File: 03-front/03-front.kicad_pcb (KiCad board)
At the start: 2 copper layers, 120 x 23.7 mm, 18 parts, among them J1 Conn_01x10

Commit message: がんばる
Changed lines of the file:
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@@
     (fp_line (start 1.6 0.8) (end -1.6 0.8)
       (stroke (width 0.1) (type solid)) (layer "F.Fab"))
-    (pad "1" smd roundrect (at -1.4625 0 270) (size 1.125 1.75) (layers "F.Cu" "F.Paste" "F.Mask") (roundrect_rratio 0.222222)
+    (pad "1" smd roundrect (at -1.4625 0 270) (size 1.125 1.75) (layers "F.Cu" "F.Paste" "F.Mask") (roundrect_rratio 0.2222222222)
       (net 1 "+3V3") (pintype "passive"))
-    (pad "2" smd roundrect (at 1.4625 0 270) (size 1.125 1.75) (layers "F.Cu" "F.Paste" "F.Mask") (roundrect_rratio 0.222222)
+    (pad "2" smd roundrect (at 1.4625 0 270) (size 1.125 1.75) (layers "F.Cu" "F.Paste" "F.Mask") (roundrect_rratio 0.2222222222)
       (net 2 "photo1") (pintype "passive"))
     (model "${KICAD6_3DMODEL_DIR}/Resistor_SMD.3dshapes/R_1206_3216Metric.wrl"
@@
     (fp_line (start 1 0.625) (end -1 0.625)
       (stroke (width 0.1) (type solid)) (layer "F.Fab"))
-    (pad "1" smd roundrect (at -0.9125 0) (size 1.025 1.4) (layers "F.Cu" "F.Paste" "F.Mask") (roundrect_rratio 0.243902)
+    (pad "1" smd roundrect (at -0.9125 0) (size 1.025 1.4) (layers "F.Cu" "F.Paste" "F.Mask") (roundrect_rratio 0.243902439)
       (net 11 "Net-(D1-A)") (pintype "passive"))
-    (pad "2" smd roundrect (at 0.9125 0) (size 1.025 1.4) (layers "F.Cu" "F.Paste" "F.Mask") (roundrect_rratio 0.243902)
+    (pad "2" smd roundrect (at 0.9125 0) (size 1.025 1.4) (layers "F.Cu" "F.Paste" "F.Mask") (roundrect_rratio 0.243902439)
       (net 1 "+3V3") (pintype "passive"))
     (model "${KICAD6_3DMODEL_DIR}/Resistor_SMD.3dshapes/R_0805_2012Metric.wrl"
@@
     (pad "9" thru_hole oval (at 0 -20.32 270) (size 1.7 1.7) (drill 1) (layers "*.Cu" "*.Mask"))
     (pad "10" thru_hole oval (at 0 -22.86 270) (size 1.7 1.7) (drill 1) (layers "*.Cu" "*.Mask"))
-    (model "${KICAD6_3DMODEL_DIR}/Connector_PinHeader_2.54mm.3dshapes/PinHeader_1x10_P2.54mm_Horizontal.wrl"
+    (model "${KICAD6_3DMODEL_DIR}/Connector_PinHeader_2.54mm.3dshapes/PinHeader_1x10_P2.54mm_Horizontal.wrl" hide
       (offset (xyz 0 0 0))
       (scale (xyz 1 1 1))
@@
     (pad "10" thru_hole oval (at 0 -22.86 270) (size 1.7 1.7) (drill 1) (layers "*.Cu" "*.Mask")
       (net 3 "GND") (pinfunction "Pin_10") (pintype "passive"))
-    (model "${KICAD6_3DMODEL_DIR}/Connector_PinHeader_2.54mm.3dshapes/PinHeader_1x10_P2.54mm_Horizontal.wrl"
+    (model "${KICAD6_3DMODEL_DIR}/Connector_PinHeader_2.54mm.3dshapes/PinHeader_1x10_P2.54mm_Horizontal.wrl" hide
       (offset (xyz 0 0 0))
       (scale (xyz 1 1 1))

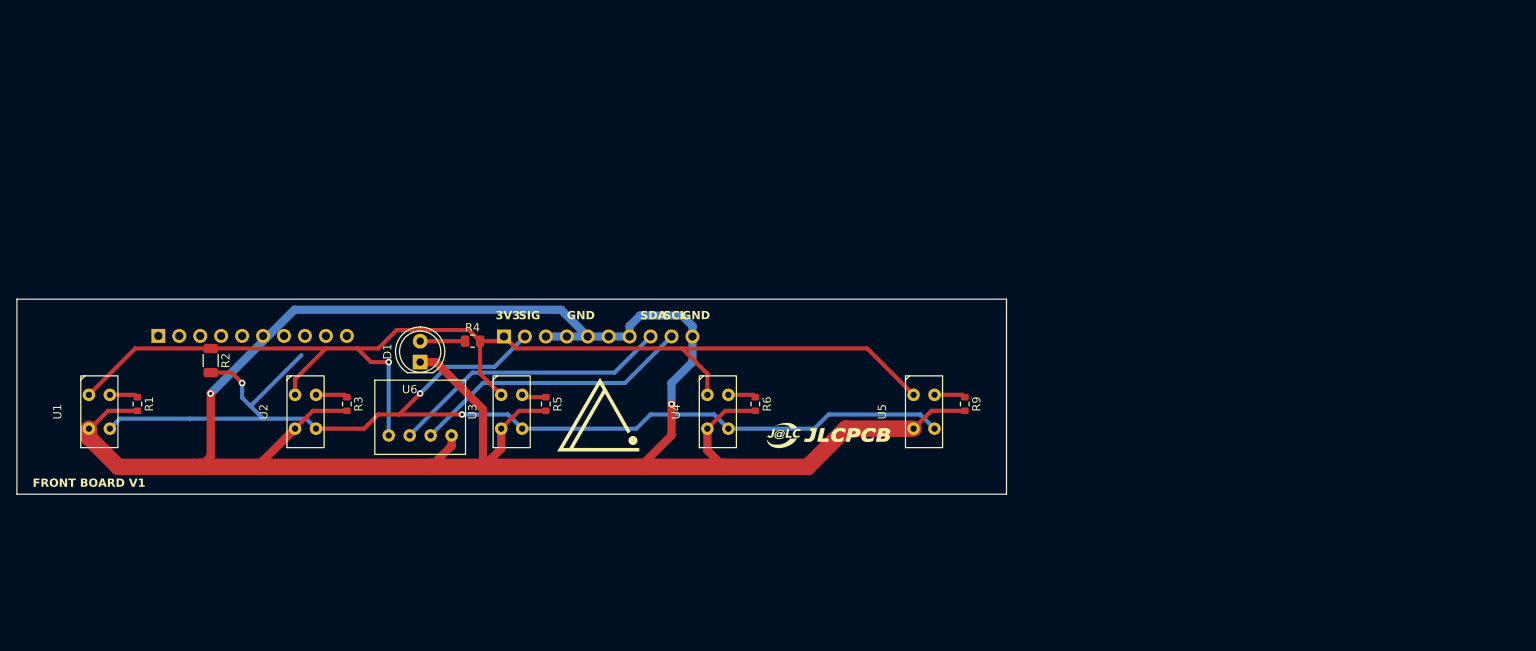
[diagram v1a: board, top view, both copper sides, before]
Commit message: わああ
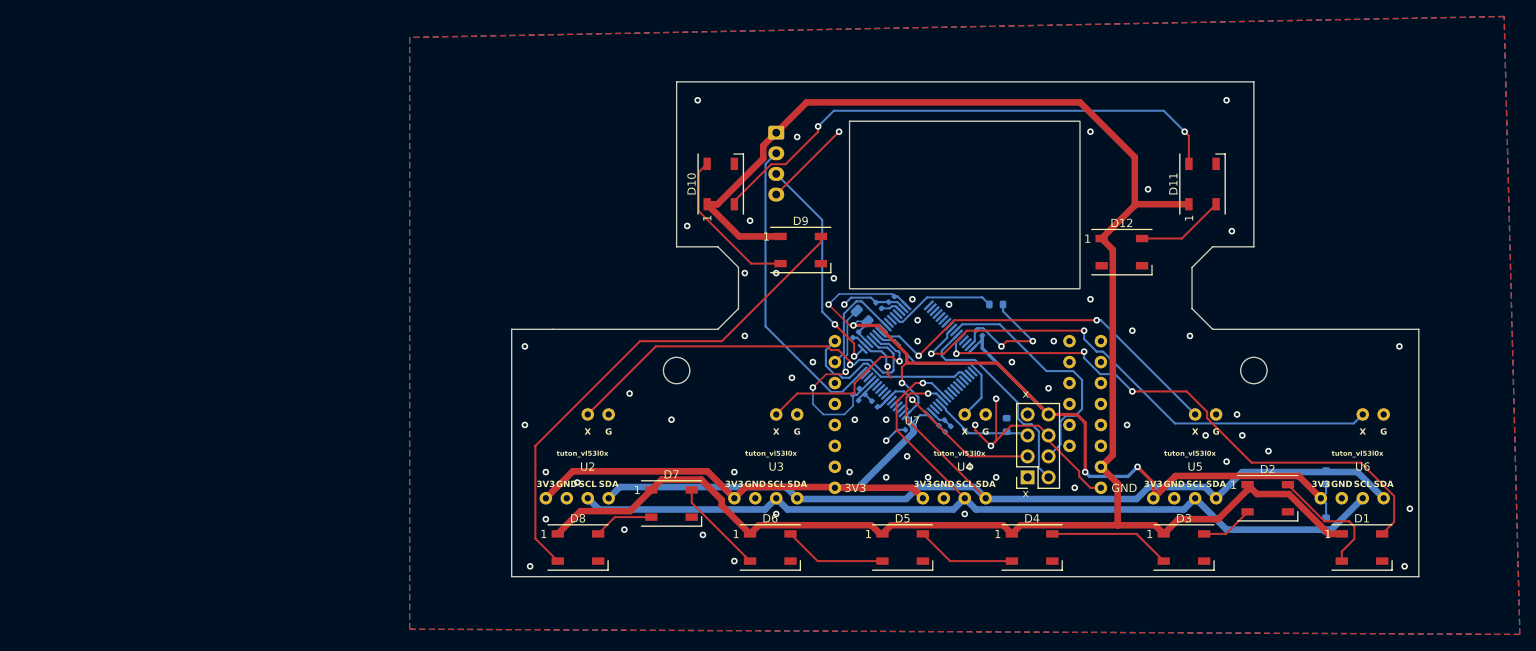
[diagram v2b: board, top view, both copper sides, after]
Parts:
- removed the G*** at (138.4, 102.9)
- removed R5, R6, R9: 105, Resistor_SMD:R_0603_1608Metric
- removed the REF** at (57.1, 90.8)
- added C1: 100n, Capacitor_SMD:C_0402_1005Metric, B.Cu at (144.0, 99.1)
- added C10: 1u, Capacitor_SMD:C_0402_1005Metric, B.Cu at (141.7, 98.3)
- added C2: 4.7u, Capacitor_SMD:C_0402_1005Metric, B.Cu at (144.5, 87.1)
- added C3: 100n, Capacitor_SMD:C_0402_1005Metric, B.Cu at (156.7, 90.4)
- added C4: 100n, Capacitor_SMD:C_0402_1005Metric, B.Cu at (141.7, 90.7)
- added C5: 100n, Capacitor_SMD:C_0402_1005Metric, B.Cu at (148.1, 101.9)
- added C6: 100n, Capacitor_SMD:C_0402_1005Metric, B.Cu at (146.1, 86.4)
- added C7: 4.7u, Capacitor_SMD:C_0402_1005Metric, B.Cu at (152.9, 102.1)
- added C8: 100n, Capacitor_SMD:C_0402_1005Metric, B.Cu at (152.1, 101.3)
- added C9: 100n, Capacitor_SMD:C_0402_1005Metric, B.Cu at (142.5, 97.5)
- added D10: WS2812B, LED_SMD:LED_WS2812B_PLCC4_5.0x5.0mm_P3.2mm, F.Cu at (125.3, 72.4)
- added D11: WS2812B, LED_SMD:LED_WS2812B_PLCC4_5.0x5.0mm_P3.2mm, F.Cu at (183.8, 72.4)
- added D12: WS2812B, LED_SMD:LED_WS2812B_PLCC4_5.0x5.0mm_P3.2mm, F.Cu at (174.0, 80.6)
- added D2: WS2812B, LED_SMD:LED_WS2812B_PLCC4_5.0x5.0mm_P3.2mm, F.Cu at (191.7, 110.5)
- added D3: WS2812B, LED_SMD:LED_WS2812B_PLCC4_5.0x5.0mm_P3.2mm, F.Cu at (181.5, 116.5)
- added D4: WS2812B, LED_SMD:LED_WS2812B_PLCC4_5.0x5.0mm_P3.2mm, F.Cu at (163.1, 116.5)
- added D5: WS2812B, LED_SMD:LED_WS2812B_PLCC4_5.0x5.0mm_P3.2mm, F.Cu at (147.4, 116.5)
- added D6: WS2812B, LED_SMD:LED_WS2812B_PLCC4_5.0x5.0mm_P3.2mm, F.Cu at (131.4, 116.5)
- added D7: WS2812B, LED_SMD:LED_WS2812B_PLCC4_5.0x5.0mm_P3.2mm, F.Cu at (119.4, 111.1)
- added D8: WS2812B, LED_SMD:LED_WS2812B_PLCC4_5.0x5.0mm_P3.2mm, F.Cu at (108.0, 116.5)
- added D9: WS2812B, LED_SMD:LED_WS2812B_PLCC4_5.0x5.0mm_P3.2mm, F.Cu at (135.1, 80.4)
- added FB1: FerriteBead, Resistor_SMD:R_0805_2012Metric, B.Cu at (142.5, 88.4)
- added G***: LOGO, logo:st_logo, B.Cu at (191.8, 108.0)
- added G***: LOGO, logo:jlcpcb_logo, B.Cu at (191.8, 104.1)
- added J2: ToMAIN, Connector_JST:JST_XH_B4B-XH-A_1x04_P2.50mm_Vertical, B.Cu at (132.1, 66.2)
- added REF**: MountingHole_3.2mm_M3, MountingHole:MountingHole_3.2mm_M3, F.Cu at (190.0, 95.0)
- added REF**: MountingHole_3.2mm_M3, MountingHole:MountingHole_3.2mm_M3, F.Cu at (120.0, 95.0)
- added U7: ~, OpenMV:OpenMV h7, F.Cu at (148.6, 101.6)
- D1: value LED -> WS2812B; footprint LED_THT:LED_D5.0mm -> LED_SMD:LED_WS2812B_PLCC4_5.0x5.0mm_P3.2mm
- G***: moved to B.Cu
- J1: value Conn_01x10 -> WRITER CONN; footprint Connector_PinHeader_2.54mm:PinHeader_1x10_P2.54mm_Horizontal -> Connector_PinSocket_2.54mm:PinSocket_2x04_P2.54mm_Vertical; moved to F.Cu
- R1, R3: value 105 -> 10k; moved to B.Cu
- R2: value 1k -> 10k; footprint Resistor_SMD:R_1206_3216Metric -> Resistor_SMD:R_0603_1608Metric; moved to B.Cu
- R4: value 100 -> 10k; footprint Resistor_SMD:R_0805_2012Metric -> Resistor_SMD:R_0603_1608Metric; moved to B.Cu
- U1: value ~ -> STM32F446RETx; footprint Akiduki:LBR127HLD -> Package_QFP:LQFP-64_10x10mm_P0.5mm; moved to B.Cu
- U2, U3, U4, U5: footprint Akiduki:LBR127HLD -> tuton:VL53L0X_horizontal
- U6: footprint S11059:S11059 -> tuton:VL53L0X_horizontal
- moved R3 119.1 mm to (198.8, 108.0), turned to 90 degrees
- moved D1 116.4 mm to (203.1, 116.5), turned to 0 degrees
- moved U6 109.5 mm to (198.1, 110.5)
- moved R4 105.9 mm to (198.8, 113.7), turned to 90 degrees
- moved R1 105.4 mm to (160.0, 101.6), turned to 90 degrees
- moved U1 99.4 mm to (149.2, 93.8), turned to 45 degrees
- moved R2 95.5 mm to (158.8, 87.0), turned to 0 degrees
- moved J1 65.8 mm to (162.6, 108.0), turned to 180 degrees
- moved U2 31.0 mm to (104.1, 110.5), turned to 0 degrees
- moved U5 29.7 mm to (177.8, 110.5), turned to 0 degrees
- moved U3 29.0 mm to (127.0, 110.5), turned to 0 degrees
- moved U4 27.0 mm to (149.9, 110.5), turned to 0 degrees
- moved G*** 11.3 mm to (119.4, 107.3), turned to 180 degrees
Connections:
- D1 pad 1: GND -> +5V
- D1 pad 2: Net-(D1-A) -> Net-(D1-DOUT)
- J1 pad 1: +3V3 -> unconnected-(J1-Pin_1-Pad1)
- J1 pad 2: photo1 -> UART1_RX
- J1 pad 3: GND -> NRST
- J1 pad 4: GND -> UART1_TX
- J1 pad 5: GND -> BOOT0
- J1 pad 7: GND -> unconnected-(J1-Pin_7-Pad7)
- J1 pad 8: SDA -> +3V3
- R1 pad 1: Net-(U1-Cathode) -> BOOT0
- R2 pad 1: +3V3 -> Net-(U1-PB2)
- R2 pad 2: photo1 -> GND
- R3 pad 1: Net-(U2-Cathode) -> +3V3
- R3 pad 2: GND -> I2C1_SDA
- R4 pad 1: Net-(D1-A) -> I2C1_SCL
- U1 pad 2: Net-(U1-Cathode) -> unconnected-(U1-PC13-Pad2)
- U1 pad 3: GND -> unconnected-(U1-PC14-Pad3)
- U1 pad 4: photo1 -> unconnected-(U1-PC15-Pad4)
- U2 pad 2: Net-(U2-Cathode) -> GND
- U2 pad 3: GND -> I2C1_SCL
- U2 pad 4: photo1 -> I2C1_SDA
- U3 pad 2: Net-(U3-Cathode) -> GND
- U3 pad 3: GND -> I2C1_SCL
- U3 pad 4: photo1 -> I2C1_SDA
- U4 pad 2: Net-(U4-Cathode) -> GND
- U4 pad 3: GND -> I2C1_SCL
- U4 pad 4: photo1 -> I2C1_SDA
- U5 pad 2: Net-(U5-Cathode) -> GND
- U5 pad 3: GND -> I2C1_SCL
- U5 pad 4: photo1 -> I2C1_SDA
- U6 pad 2: SDA -> GND
- U6 pad 3: SCL -> I2C1_SCL
- U6 pad 4: GND -> I2C1_SDA
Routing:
- net +5V: track 0.00 -> 234.9 mm
- net GND: track 278.1 -> 80.3 mm, vias 2 -> 65
- net photo1: track 142.9 -> 0.00 mm, vias 3 -> 0
- net I2C1_SCL: track 0.00 -> 123.3 mm, vias 0 -> 1
- net I2C1_SDA: track 0.00 -> 121.4 mm, vias 0 -> 1
- net WS2812B: track 0.00 -> 68.8 mm, vias 0 -> 3
- net Net-(D10-DOUT): track 0.00 -> 65.1 mm, vias 0 -> 2
- net XSHUT5: track 0.00 -> 63.3 mm, vias 0 -> 2
- net Net-(D8-DOUT): track 0.00 -> 60.7 mm
- net +3V3: track 142.0 -> 192.2 mm, vias 1 -> 5
- net XSHUT1: track 0.00 -> 48.0 mm, vias 0 -> 1
- net XSHUT4: track 0.00 -> 45.9 mm, vias 0 -> 2
- net UART2_TX: track 0.00 -> 37.6 mm
- net SDA: track 34.2 -> 0.00 mm
- net SCL: track 34.2 -> 0.00 mm
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- added copper zone on B.Cu, net GND
- added copper zone on F.Cu, net GND
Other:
- board size 120 x 23.7 mm -> 110 x 60 mm
- board text added: "03-front ver.1"
- board text added: "1"
- board text added: "5V"
- board text added: "RCJ 2025 tuton"
- board text added: "front→main"
- board text added: "main→front"
- board text added: "x"
- board text removed: "FRONT BOARD V1"
- board text removed: "SCL"
- board text removed: "SDA"
- board text removed: "SIG"
